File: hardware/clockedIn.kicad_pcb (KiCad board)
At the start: 2 copper layers, 24 parts, among them SW1 SW_SPDT, U1 TPIC6B595N, U2 TPIC6B595N, U3 TPIC6B595N, U4 TPIC6B595N, U5 TPIC6B595N, U6 TPIC6B595N, U7 TPIC6B595N, U8 TPIC6B595N, U9 TPIC6B595N

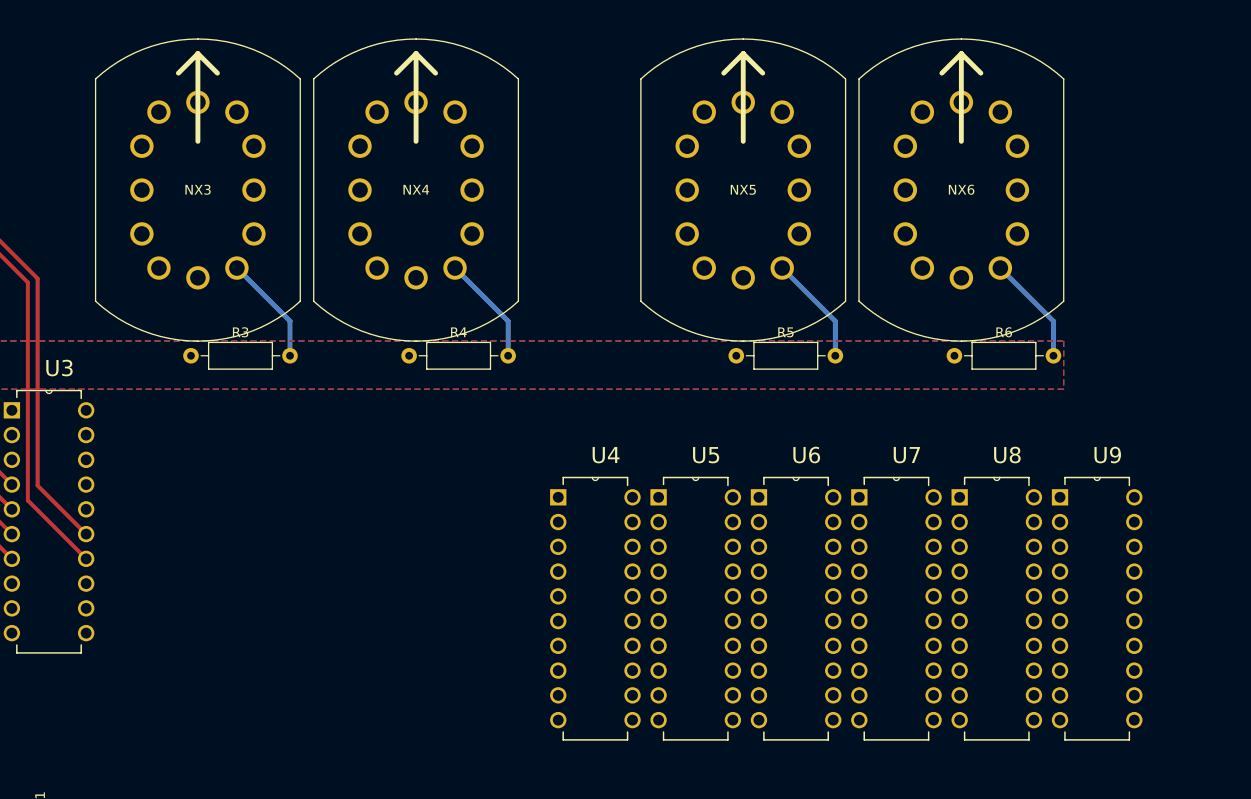
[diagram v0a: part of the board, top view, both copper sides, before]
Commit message: hardwareisveryhard
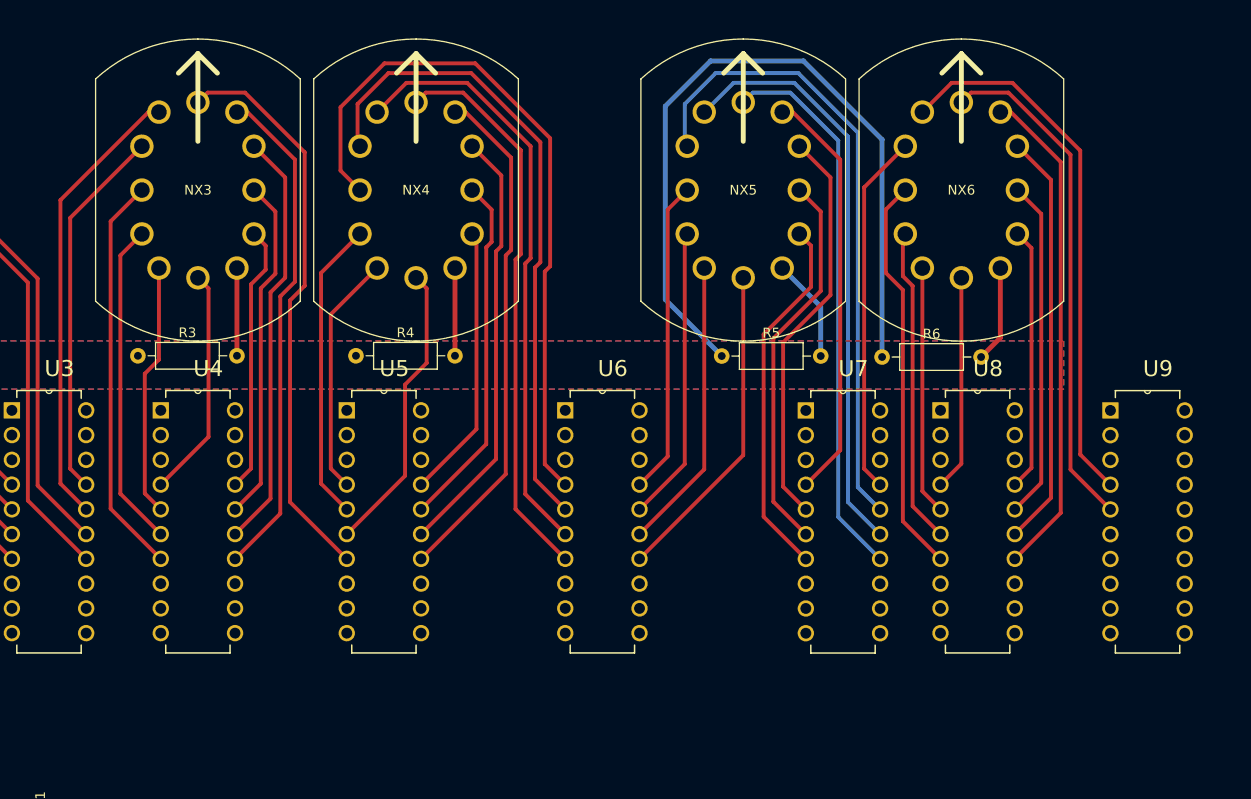
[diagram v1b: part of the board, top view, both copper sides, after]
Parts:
- moved U4 41.7 mm to (97.3, 76.5)
- moved U5 33.2 mm to (116.4, 76.5)
- moved U6 21.8 mm to (138.8, 76.5)
- moved U7 10.5 mm to (163.5, 76.5)
- moved U9 10.3 mm to (194.7, 76.5)
- moved U8 9.14 mm to (177.3, 76.5)
- moved R6 7.43 mm to (163.7, 48.1)
- moved R4 5.45 mm to (109.7, 48.0)
- moved R3 5.44 mm to (87.3, 48.0)
- moved R5 1.50 mm to (147.2, 48.0)
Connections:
- NX3 pad 0: unconnected-(NX3-Pad0) -> /C0
- NX3 pad 1: unconnected-(NX3-Pad1) -> /C1
- NX3 pad 2: unconnected-(NX3-Pad2) -> /C2
- NX3 pad 3: unconnected-(NX3-Pad3) -> /C3
- NX3 pad 4: unconnected-(NX3-Pad4) -> /C4
- NX3 pad 5: unconnected-(NX3-Pad5) -> /C5
- NX3 pad 6: unconnected-(NX3-Pad6) -> /C6
- NX3 pad 7: unconnected-(NX3-Pad7) -> /C7
- NX3 pad 8: unconnected-(NX3-Pad8) -> /C8
- NX3 pad 9: unconnected-(NX3-Pad9) -> /C9
- NX3 pad LHDP: unconnected-(NX3-PadLHDP) -> /C.
- NX4 pad 0: unconnected-(NX4-Pad0) -> /D0
- NX4 pad 1: unconnected-(NX4-Pad1) -> /D1
- NX4 pad 2: unconnected-(NX4-Pad2) -> /D2
- NX4 pad 3: unconnected-(NX4-Pad3) -> /D3
- NX4 pad 4: unconnected-(NX4-Pad4) -> /D4
- NX4 pad 5: unconnected-(NX4-Pad5) -> /D5
- NX4 pad 6: unconnected-(NX4-Pad6) -> /D6
- NX4 pad 7: unconnected-(NX4-Pad7) -> /D7
- NX4 pad 8: unconnected-(NX4-Pad8) -> /D8
- NX4 pad 9: unconnected-(NX4-Pad9) -> /D9
- NX4 pad LHDP: unconnected-(NX4-PadLHDP) -> /D.
- NX5 pad 0: unconnected-(NX5-Pad0) -> /E0
- NX5 pad 1: unconnected-(NX5-Pad1) -> /E1
- NX5 pad 2: unconnected-(NX5-Pad2) -> /E2
- NX5 pad 3: unconnected-(NX5-Pad3) -> /E3
- NX5 pad 4: unconnected-(NX5-Pad4) -> /E4
- NX5 pad 5: unconnected-(NX5-Pad5) -> /E5
- NX5 pad 6: unconnected-(NX5-Pad6) -> /E6
- NX5 pad 7: unconnected-(NX5-Pad7) -> /E7
- NX5 pad 8: unconnected-(NX5-Pad8) -> /E8
- NX5 pad 9: unconnected-(NX5-Pad9) -> /E9
- NX5 pad LHDP: unconnected-(NX5-PadLHDP) -> /E.
- NX6 pad 0: unconnected-(NX6-Pad0) -> /F0
- NX6 pad 1: unconnected-(NX6-Pad1) -> /F1
- NX6 pad 2: unconnected-(NX6-Pad2) -> /F2
- NX6 pad 3: unconnected-(NX6-Pad3) -> /F3
- NX6 pad 4: unconnected-(NX6-Pad4) -> /F4
- NX6 pad 5: unconnected-(NX6-Pad5) -> /F5
- NX6 pad 6: unconnected-(NX6-Pad6) -> /F6
- NX6 pad 7: unconnected-(NX6-Pad7) -> /F7
- NX6 pad 8: unconnected-(NX6-Pad8) -> /F8
- NX6 pad 9: unconnected-(NX6-Pad9) -> /F9
- NX6 pad LHDP: unconnected-(NX6-PadLHDP) -> /F.
- U3 pad 16: unconnected-(U3-DRAIN6-Pad16) -> /C5
- U3 pad 17: unconnected-(U3-DRAIN7-Pad17) -> /C4
- U4 pad 14: unconnected-(U4-DRAIN4-Pad14) -> /C7
- U4 pad 15: unconnected-(U4-DRAIN5-Pad15) -> /C8
- U4 pad 16: unconnected-(U4-DRAIN6-Pad16) -> /C9
- U4 pad 17: unconnected-(U4-DRAIN7-Pad17) -> /C0
- U4 pad 4: unconnected-(U4-DRAIN0-Pad4) -> /C.
- U4 pad 5: unconnected-(U4-DRAIN1-Pad5) -> /C1
- U4 pad 6: unconnected-(U4-DRAIN2-Pad6) -> /C2
- U4 pad 7: unconnected-(U4-DRAIN3-Pad7) -> /C3
- U5 pad 14: unconnected-(U5-DRAIN4-Pad14) -> /D7
- U5 pad 15: unconnected-(U5-DRAIN5-Pad15) -> /D8
- U5 pad 16: unconnected-(U5-DRAIN6-Pad16) -> /D9
- U5 pad 17: unconnected-(U5-DRAIN7-Pad17) -> /D0
- U5 pad 4: unconnected-(U5-DRAIN0-Pad4) -> /D1
- U5 pad 5: unconnected-(U5-DRAIN1-Pad5) -> /D2
- U5 pad 6: unconnected-(U5-DRAIN2-Pad6) -> /D.
- U5 pad 7: unconnected-(U5-DRAIN3-Pad7) -> /C6
- U6 pad 14: unconnected-(U6-DRAIN4-Pad14) -> /E.
- U6 pad 15: unconnected-(U6-DRAIN5-Pad15) -> /E1
- U6 pad 16: unconnected-(U6-DRAIN6-Pad16) -> /E2
- U6 pad 17: unconnected-(U6-DRAIN7-Pad17) -> /E3
- U6 pad 4: unconnected-(U6-DRAIN0-Pad4) -> /D3
- U6 pad 5: unconnected-(U6-DRAIN1-Pad5) -> /D4
- U6 pad 6: unconnected-(U6-DRAIN2-Pad6) -> /D5
- U6 pad 7: unconnected-(U6-DRAIN3-Pad7) -> /D6
- U7 pad 14: unconnected-(U7-DRAIN4-Pad14) -> /E6
- U7 pad 15: unconnected-(U7-DRAIN5-Pad15) -> /E5
- U7 pad 16: unconnected-(U7-DRAIN6-Pad16) -> /E4
- U7 pad 17: unconnected-(U7-DRAIN7-Pad17) -> /F4
- U7 pad 4: unconnected-(U7-DRAIN0-Pad4) -> /E7
- U7 pad 5: unconnected-(U7-DRAIN1-Pad5) -> /E8
- U7 pad 6: unconnected-(U7-DRAIN2-Pad6) -> /E9
- U7 pad 7: unconnected-(U7-DRAIN3-Pad7) -> /E0
- U8 pad 14: unconnected-(U8-DRAIN4-Pad14) -> /F7
- U8 pad 15: unconnected-(U8-DRAIN5-Pad15) -> /F8
- U8 pad 16: unconnected-(U8-DRAIN6-Pad16) -> /F9
- U8 pad 17: unconnected-(U8-DRAIN7-Pad17) -> /F0
- U8 pad 4: unconnected-(U8-DRAIN0-Pad4) -> /F.
- U8 pad 5: unconnected-(U8-DRAIN1-Pad5) -> /F1
- U8 pad 6: unconnected-(U8-DRAIN2-Pad6) -> /F2
- U8 pad 7: unconnected-(U8-DRAIN3-Pad7) -> /F3
- U9 pad 4: unconnected-(U9-DRAIN0-Pad4) -> /F5
- U9 pad 5: unconnected-(U9-DRAIN1-Pad5) -> /F6
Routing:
- net 170v: track 0.00 -> 77.9 mm
- net /D3: track 0.00 -> 72.5 mm
- net /D4: track 0.00 -> 66.6 mm
- net /E4: track 0.00 -> 65.6 mm
- net /D5: track 0.00 -> 61.4 mm
- net /E5: track 0.00 -> 60.4 mm
- net /C6: track 0.00 -> 58.7 mm
- net /D6: track 0.00 -> 57.9 mm
- net /E6: track 0.00 -> 56.9 mm
- net /F5: track 0.00 -> 55.9 mm
- net /D7: track 0.00 -> 52.7 mm
- net /F6: track 0.00 -> 52.3 mm
- net /C7: track 0.00 -> 51.5 mm
- net /F7: track 0.00 -> 51.0 mm
- net /C5: track 0.00 -> 46.7 mm
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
